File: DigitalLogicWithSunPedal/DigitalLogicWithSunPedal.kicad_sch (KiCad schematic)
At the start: 23 parts, among them IC1 REG1117-5, IC2 74LS08, J1 776280-1, J2 4pin brake, J3 4pin throttle, K1 J107F1AS123VDC.36, Q1 2N2222A, U2 TS881ICT, U3 TS881ICT, U4 TS881ICT, U5 TS881ICT

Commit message: Add files via upload
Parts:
- removed C1, C2: C, symbol Device:C
- removed R1, R2, R3, R4, R5, R6: R_US, symbol Device:R_US
- added C1, C2: CL21A106KOQNNNE, CL21A106KOQNNNE:CAPC2012X140N, symbol CL21A106KOQNNNE:CL21A106KOQNNNE
- added R10, R11, R12, R7, R8, R9: CRCW08051K00FKEA, CRCW08051K00FKEA:RESC2012X50N, symbol CRCW08051K00FKEA:CRCW08051K00FKEA
- #J3, #J4: value DT15-4P (4 pin connector for the brake & throttle port) -> DT15-4P
- IC2: value 74LS08 -> HEF4081BT,653; footprint 74LS08:DIL14 -> Package_SO:SOIC-14_3.9x8.7mm_P1.27mm
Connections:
- net +12V: now also C1.1; no longer J1.4, J2.2, U4.3 (+), U5.3 (+)
- net +5V: now also C2.1
- net GND: now also C1.2, C2.2, R10.2, R11.2, R12.2, R7.2, R8.2, R9.2
- net at IC2.10, IC2.6: now also R9.1
- net at IC2.3, IC2.9: now also R10.1
- net at IC2.5, U4.1: now also R7.1
- net at IC2.4, U5.1: now also R8.1
- net at IC2.1, U2.1: now also R12.1
- net at IC2.2, U3.1: now also R11.1
- new net: J1.4, J2.2, U4.3 (+), U5.3 (+)
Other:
- moved on the sheet: IC1, IC2A, IC2B, IC2C, IC2D, IC2E, J1, K1, Q1, U2, U3, U4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

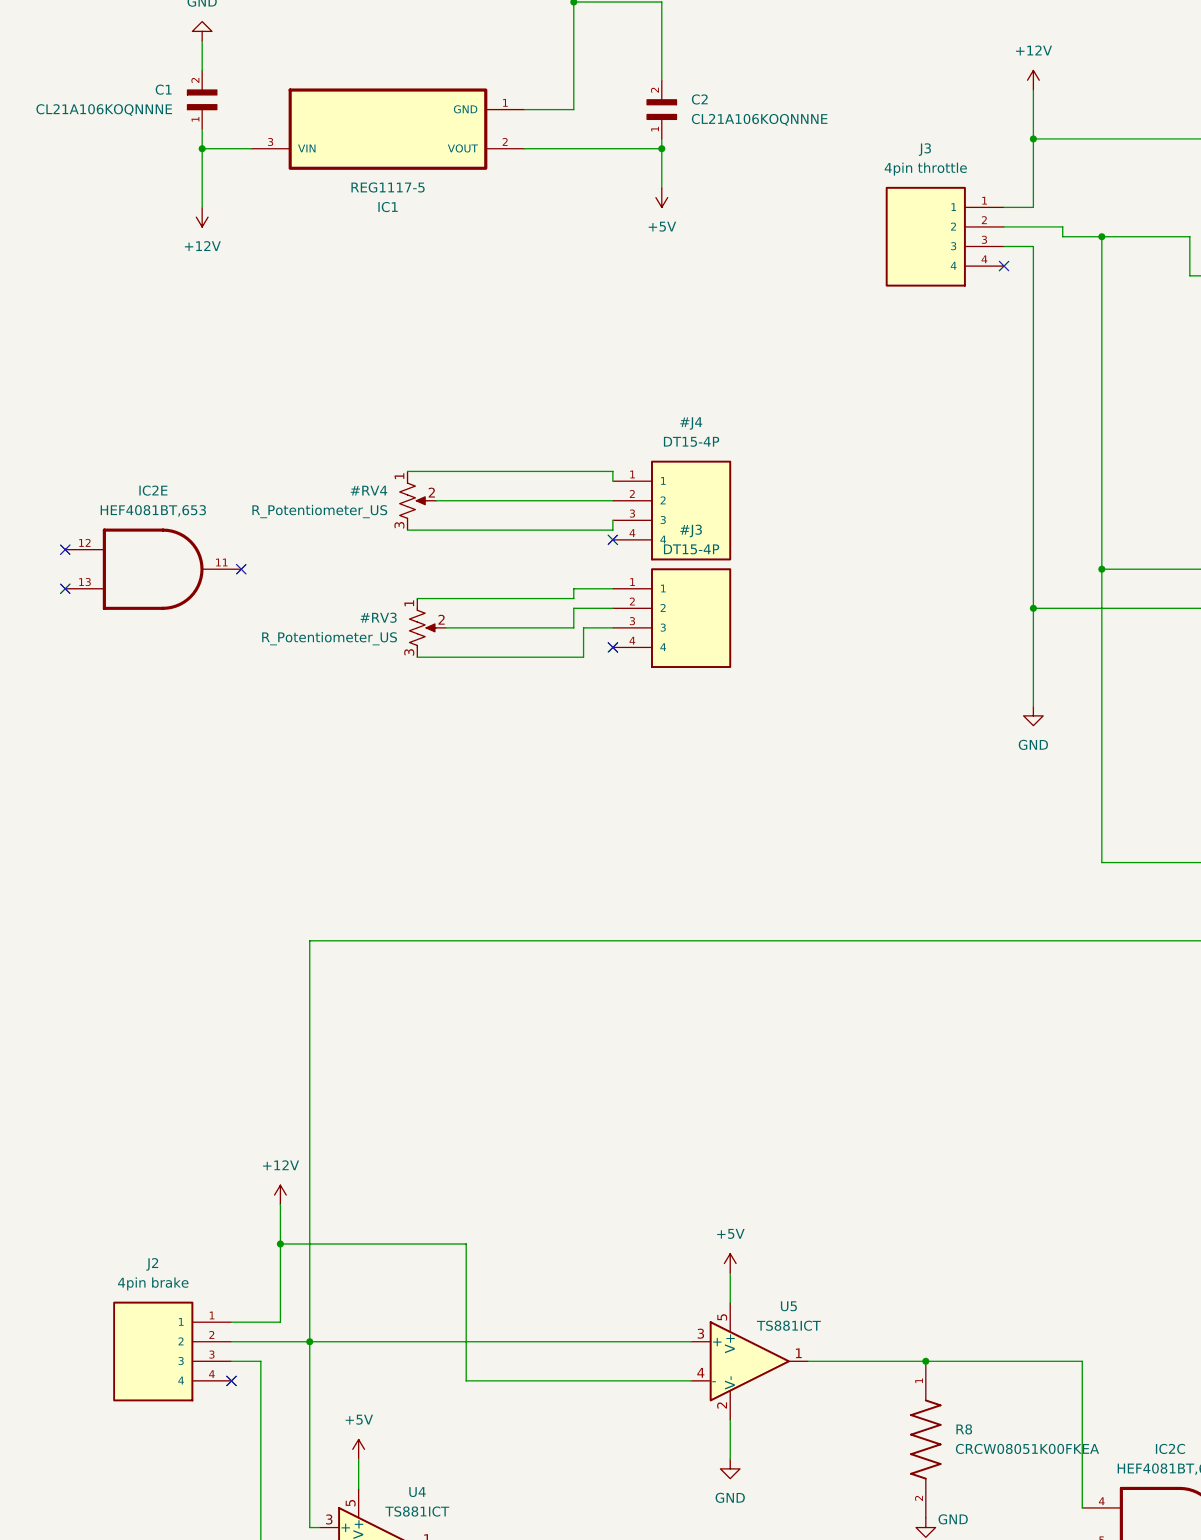
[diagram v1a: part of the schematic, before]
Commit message: Add files via upload
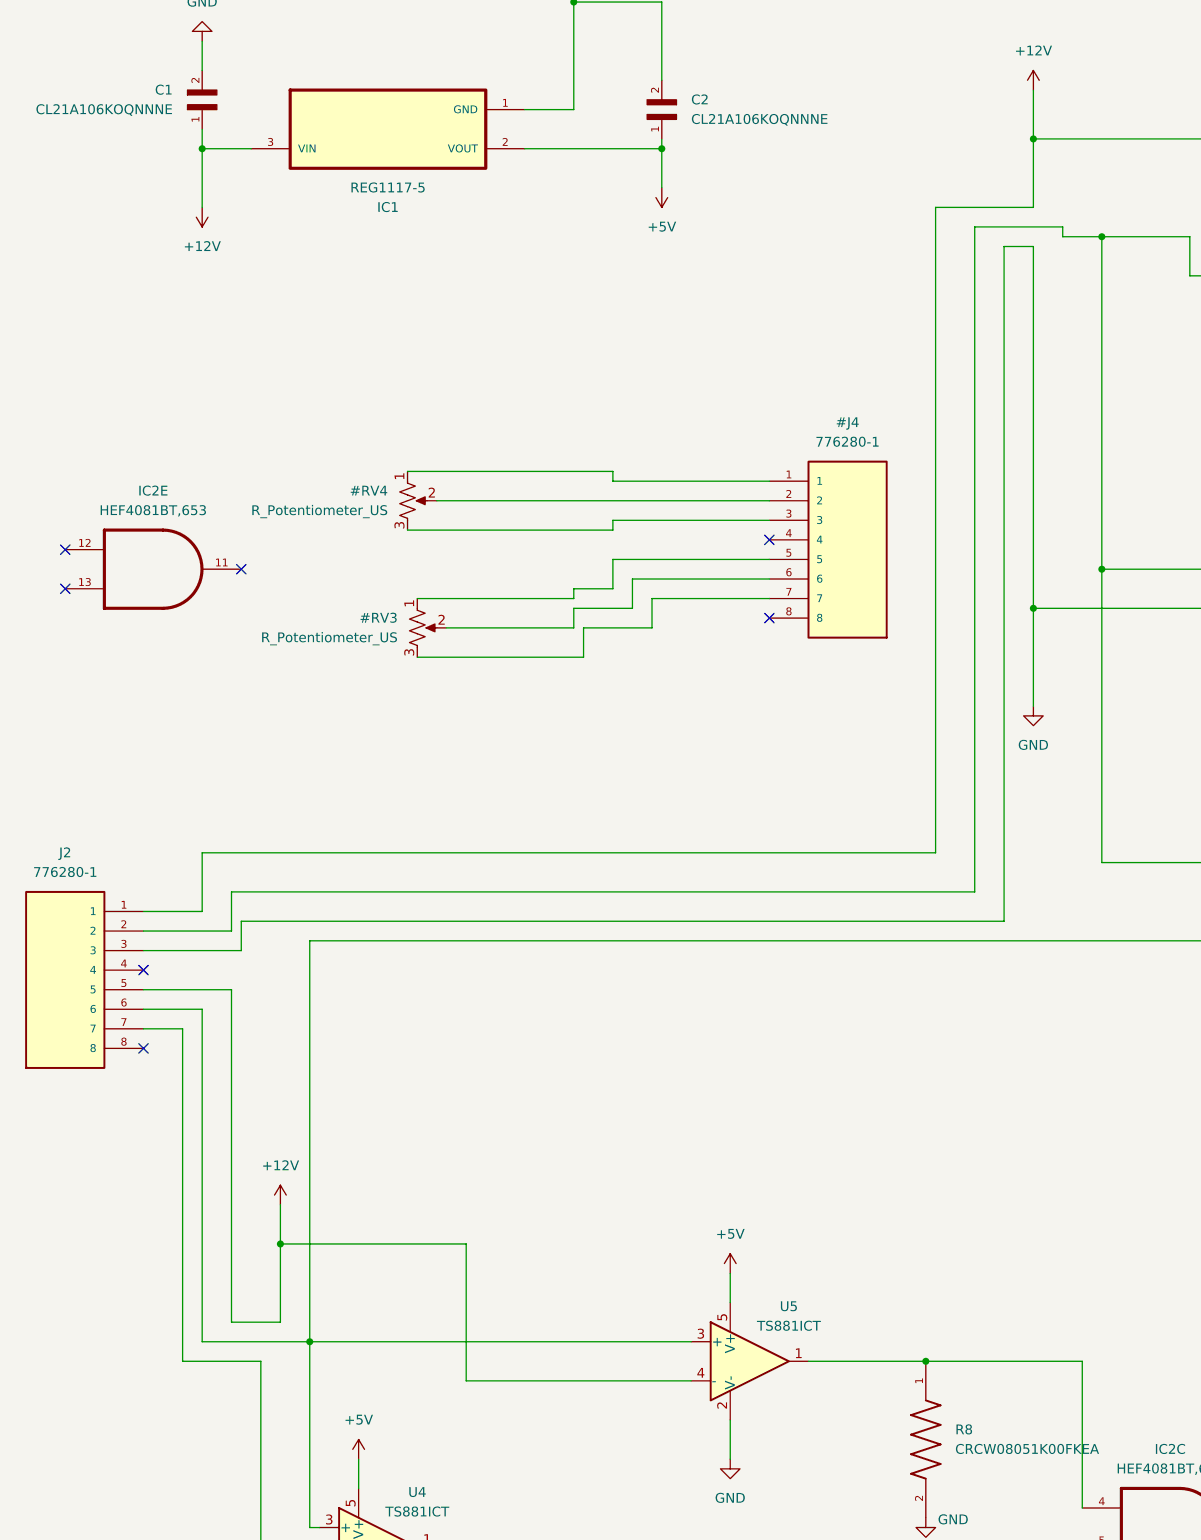
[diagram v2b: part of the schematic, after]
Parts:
- removed #J3, #J4: DT15-4P, DT15-4P:TE_DT15-4P, symbol DT15-4P:DT15-4P
- removed J2: 4pin brake, DT15-4P:TE_DT15-4P, symbol DT15-4P:DT15-4P
- removed J3: 4pin throttle, DT15-4P:TE_DT15-4P, symbol DT15-4P:DT15-4P
- added #J4, J2: 776280-1, 776280-1:TE_776280-1, symbol 776280-1:776280-1
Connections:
- net +12V: now also J2.1, J2.5
- net GND: now also J2.3, J2.7
- net at #RV3.1: now also #J4.5
- net at #RV3.2: now also #J4.6
- net at #RV3.3: now also #J4.7
- net at #RV4.1: now also #J4.1
- net at #RV4.2: now also #J4.2
- net at #RV4.3: now also #J4.3
- net at J1.4, U4.3 (+), U5.3 (+): now also J2.6
- net at J1.3, U2.4 (-), U3.3 (+): now also J2.2
